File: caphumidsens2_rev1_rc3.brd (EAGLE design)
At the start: 110 x 10 mm, 12 parts, among them IC1 ATtiny25/45/85

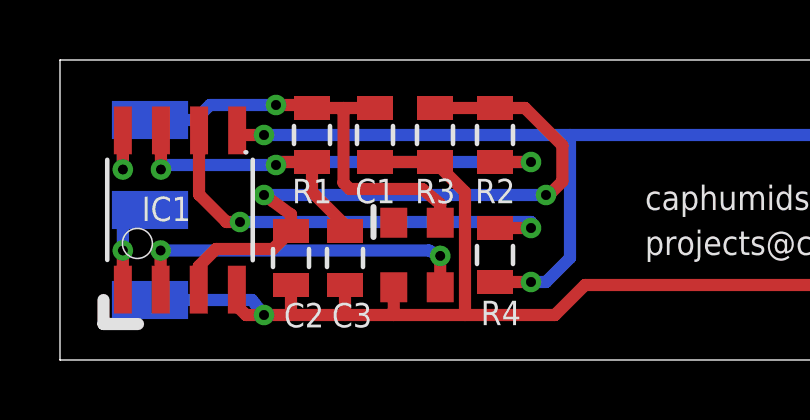
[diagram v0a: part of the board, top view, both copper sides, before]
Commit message: finetuning, misc
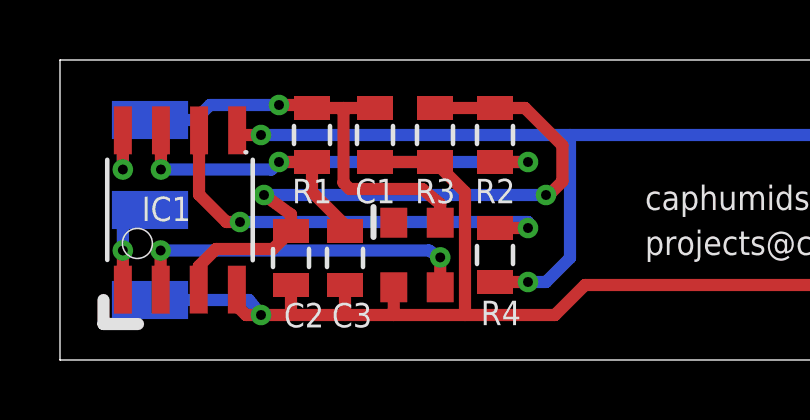
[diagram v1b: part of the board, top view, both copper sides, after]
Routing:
- net 2_3RD_VCC_VREF: track 19.3 -> 18.6 mm
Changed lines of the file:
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@@
 <wire x1="8.4" y1="8.4" x2="9.45" y2="8.4" width="0.4064" layer="1"/>
 <wire x1="8.4" y1="8.4" x2="7.9" y2="8.5" width="0.4064" layer="1"/>
-<wire x1="7.9" y1="8.5" x2="7.2" y2="8.5" width="0.4064" layer="1"/>
-<via x="7.2" y="8.5" extent="1-16" drill="0.3302"/>
+<wire x1="7.9" y1="8.5" x2="7.3" y2="8.5" width="0.4064" layer="1"/>
+<via x="7.3" y="8.5" extent="1-16" drill="0.3302"/>
 <contactref element="OSC1" pad="4"/>
 <contactref element="OSC1" pad="4"/>
@@
 <wire x1="3" y1="8" x2="4.5" y2="8" width="0.4064" layer="16"/>
 <wire x1="4.5" y1="8" x2="5" y2="8.5" width="0.4064" layer="16"/>
-<wire x1="5" y1="8.5" x2="7.2" y2="8.5" width="0.4064" layer="16"/>
+<wire x1="5" y1="8.5" x2="7.3" y2="8.5" width="0.4064" layer="16"/>
 <wire x1="12.675" y1="4.575" x2="12.675" y2="5.2" width="0.4064" layer="1"/>
 <wire x1="12.675" y1="5.2" x2="12.075" y2="5.7" width="0.4064" layer="1"/>
@@
 <wire x1="12.5" y1="6.6" x2="13.5" y2="5.6" width="0.4064" layer="1"/>
 <wire x1="13.5" y1="5.6" x2="13.5" y2="1.5" width="0.4064" layer="1"/>
-<wire x1="6.2" y1="1.5" x2="6.8" y2="1.5" width="0.4064" layer="1"/>
+<wire x1="6.2" y1="1.5" x2="6.7" y2="1.5" width="0.4064" layer="1"/>
 <wire x1="7.7" y1="1.5" x2="9.5" y2="1.5" width="0.4064" layer="1"/>
-<wire x1="6.8" y1="1.5" x2="7.7" y2="1.5" width="0.4064" layer="1"/>
+<wire x1="6.7" y1="1.5" x2="7.7" y2="1.5" width="0.4064" layer="1"/>
 <wire x1="9.5" y1="1.5" x2="11.125" y2="1.5" width="0.4064" layer="1"/>
 <wire x1="11.125" y1="1.5" x2="13.5" y2="1.5" width="0.4064" layer="1"/>
 <wire x1="6.2" y1="1.5" x2="5.895" y2="1.805" width="0.4064" layer="1"/>
-<wire x1="3" y1="2" x2="6.4" y2="2" width="0.4064" layer="16"/>
-<wire x1="6.4" y1="2" x2="6.8" y2="1.5" width="0.4064" layer="16"/>
-<via x="6.8" y="1.5" extent="1-16" drill="0.3302"/>
+<wire x1="3" y1="2" x2="6.3" y2="2" width="0.4064" layer="16"/>
+<wire x1="6.3" y1="2" x2="6.7" y2="1.5" width="0.4064" layer="16"/>
+<via x="6.7" y="1.5" extent="1-16" drill="0.3302"/>
 <wire x1="11.125" y1="2.425" x2="11.125" y2="1.5" width="0.4064" layer="1"/>
 <contactref element="IC1" pad="4"/>
@@
 <wire x1="8.4" y1="5.6" x2="9.5" y2="4.5" width="0.4064" layer="1"/>
 <wire x1="9.5" y1="4.5" x2="9.5" y2="4.3" width="0.4064" layer="1"/>
-<wire x1="7.2" y1="6.5" x2="7.1" y2="6.6" width="0.4064" layer="16"/>
-<wire x1="7.1" y1="6.6" x2="15.7" y2="6.6" width="0.4064" layer="16"/>
-<wire x1="14.5" y1="6.6" x2="15.7" y2="6.6" width="0.4064" layer="1"/>
-<via x="15.7" y="6.6" extent="1-16" drill="0.3302"/>
-<via x="7.2" y="6.5" extent="1-16" drill="0.3302"/>
+<wire x1="7.3" y1="6.6" x2="15.6" y2="6.6" width="0.4064" layer="16"/>
+<wire x1="14.5" y1="6.6" x2="15.6" y2="6.6" width="0.4064" layer="1"/>
+<via x="15.6" y="6.6" extent="1-16" drill="0.3302"/>
+<via x="7.3" y="6.6" extent="1-16" drill="0.3302"/>
 <wire x1="8.4" y1="5.6" x2="8.4" y2="6.6" width="0.4064" layer="1"/>
-<wire x1="7.2" y1="6.5" x2="7.1" y2="6.6" width="0.4064" layer="1"/>
-<wire x1="7.1" y1="6.6" x2="8.4" y2="6.6" width="0.4064" layer="1"/>
-<wire x1="3.365" y1="6.35" x2="3.565" y2="6.5" width="0.4064" layer="16"/>
-<wire x1="3.565" y1="6.5" x2="7.2" y2="6.5" width="0.4064" layer="16"/>
+<wire x1="3.365" y1="6.35" x2="7.05" y2="6.35" width="0.4064" layer="16"/>
+<wire x1="7.05" y1="6.35" x2="7.3" y2="6.6" width="0.4064" layer="16"/>
+<wire x1="7.3" y1="6.6" x2="8.4" y2="6.6" width="0.4064" layer="1"/>
 </signal>
 <signal name="1_3RD_VCC_VREF">
@@
 <vertex x="99" y="9"/>
 </polygon>
-<wire x1="6.8" y1="7.5" x2="17" y2="7.5" width="0.4064" layer="16"/>
+<wire x1="6.7" y1="7.5" x2="17" y2="7.5" width="0.4064" layer="16"/>
 <wire x1="17" y1="7.5" x2="37" y2="7.5" width="0.4064" layer="16"/>
-<via x="6.8" y="7.5" extent="1-16" drill="0.3302"/>
+<via x="6.7" y="7.5" extent="1-16" drill="0.3302"/>
 <contactref element="R4" pad="1"/>
 <wire x1="17" y1="3.4" x2="17" y2="7.5" width="0.4064" layer="16"/>
-<wire x1="6.8" y1="7.5" x2="5.905" y2="7.5" width="0.4064" layer="1"/>
+<wire x1="6.7" y1="7.5" x2="5.905" y2="7.5" width="0.4064" layer="1"/>
 <wire x1="5.905" y1="7.5" x2="5.905" y2="7.654" width="0.4064" layer="1"/>
-<via x="15.7" y="2.6" extent="1-16" drill="0.3302"/>
-<wire x1="15.7" y1="2.6" x2="14.5" y2="2.6" width="0.4064" layer="1"/>
+<via x="15.6" y="2.6" extent="1-16" drill="0.3302"/>
+<wire x1="15.6" y1="2.6" x2="14.5" y2="2.6" width="0.4064" layer="1"/>
 <wire x1="17" y1="3.4" x2="16.2" y2="2.6" width="0.4064" layer="16"/>
-<wire x1="16.2" y1="2.6" x2="15.7" y2="2.6" width="0.4064" layer="16"/>
+<wire x1="16.2" y1="2.6" x2="15.6" y2="2.6" width="0.4064" layer="16"/>
 </signal>
 <signal name="CLOCK_IN">
@@
 <via x="3.355" y="3.65" extent="1-16" drill="0.3302"/>
 <wire x1="3.355" y1="2.346" x2="3.355" y2="3.65" width="0.4064" layer="1"/>
-<via x="12.675" y="3.47" extent="1-16" drill="0.3302"/>
-<wire x1="12.675" y1="3.47" x2="12.3" y2="3.65" width="0.4064" layer="16"/>
+<via x="12.675" y="3.42" extent="1-16" drill="0.3302"/>
+<wire x1="12.675" y1="3.42" x2="12.3" y2="3.65" width="0.4064" layer="16"/>
 <wire x1="12.3" y1="3.65" x2="3.355" y2="3.65" width="0.4064" layer="16"/>
-<wire x1="12.675" y1="3.47" x2="12.675" y2="2.425" width="0.4064" layer="1"/>
+<wire x1="12.675" y1="3.42" x2="12.675" y2="2.425" width="0.4064" layer="1"/>
 </signal>
 <signal name="OUTPUT_OR_DEBUGWIRE">
@@
 <contactref element="IC1" pad="6"/>
 <contactref element="R4" pad="2"/>
-<wire x1="15.7" y1="4.6" x2="6" y2="4.6" width="0.4064" layer="16"/>
-<wire x1="14.5" y1="4.4" x2="15.7" y2="4.4" width="0.4064" layer="1"/>
-<via x="15.7" y="4.4" extent="1-16" drill="0.3302"/>
-<wire x1="15.7" y1="4.4" x2="15.7" y2="4.6" width="0.4064" layer="16"/>
+<wire x1="15.6" y1="4.6" x2="6" y2="4.6" width="0.4064" layer="16"/>
+<wire x1="14.5" y1="4.4" x2="15.6" y2="4.4" width="0.4064" layer="1"/>
+<via x="15.6" y="4.4" extent="1-16" drill="0.3302"/>
+<wire x1="15.6" y1="4.4" x2="15.6" y2="4.6" width="0.4064" layer="16"/>
 <wire x1="6" y1="4.6" x2="5.54890625" y2="4.6" width="0.4064" layer="1"/>
 <wire x1="5.54890625" y1="4.6" x2="4.635" y2="5.51390625" width="0.4064" layer="1"/>
